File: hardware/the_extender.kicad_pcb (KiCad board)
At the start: 4 copper layers, 51.2 x 50.9 mm, 119 parts, among them J0 U262-241N-4BV60, J1 USB_C_Receptacle_USB2.0, J2 U231-091N-3BLRC11, J3 PJ-3136-B, J4 PJ-3136-B, J5 AF 10.0 HC6.3, Q1 SSM3J332R,LF, Q2 SSM3J332R,LF, Q3 Q_PNP_CBE, Q4 SSM3J332R,LF, U0 RT6150BGQW, U1 IP5310, U2 RP2040, U3 W25Q32JVSS, U4 FUSB302BMPX, U5 USB2514B_Bi, U6 HS-100B, Y1 ABLS-12.000MHZ-20-B-3-H-T

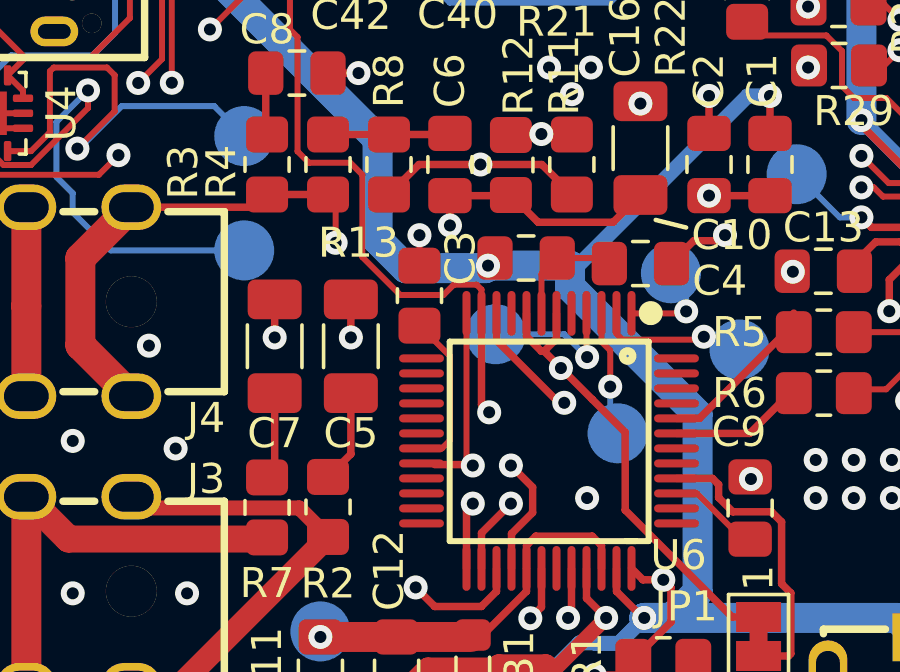
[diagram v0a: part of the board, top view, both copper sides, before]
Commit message: stuff
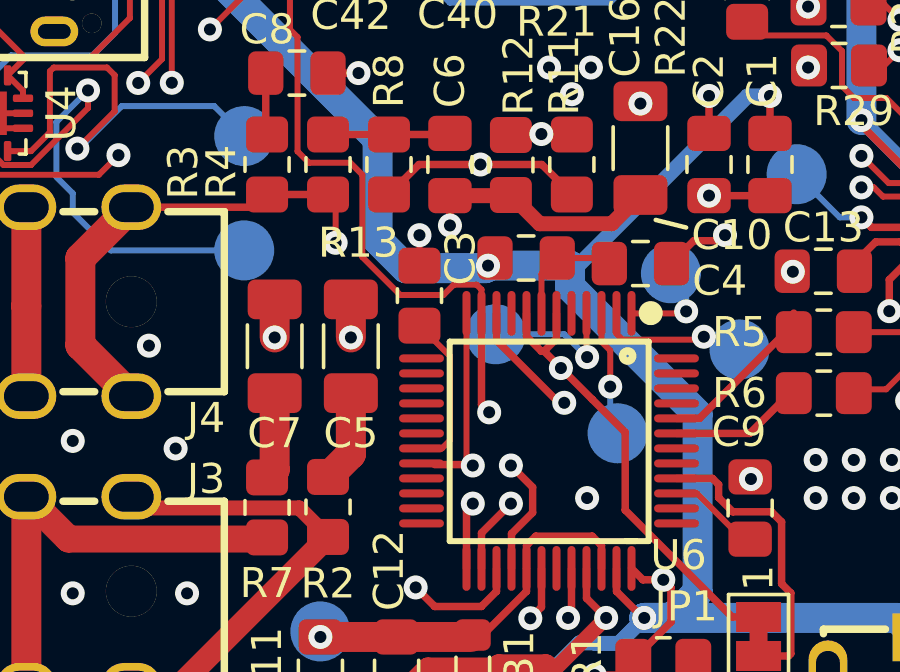
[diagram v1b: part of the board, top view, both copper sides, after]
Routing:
- net Net-(C10-Pad1): track 24.1 -> 26.4 mm
- net SND_L: track 16.0 -> 16.6 mm
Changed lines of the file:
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@@
   (segment (start 69.215 69.4) (end 69.33 69.285) (width 0.25) (layer "F.Cu") (net 5))
   (segment (start 69.33 69.285) (end 69.33 67.75) (width 0.25) (layer "F.Cu") (net 5))
-  (segment (start 61.976 60.052) (end 61.976 58.782) (width 0.25) (layer "F.Cu") (net 5))
+  (segment (start 61.976 60.052) (end 61.976 58.782) (width 1) (layer "F.Cu") (net 5))
   (via (at 61.976 60.052) (size 0.8) (drill 0.4) (layers "F.Cu" "B.Cu") (free) (net 5))
   (via (at 69.215 69.4) (size 0.8) (drill 0.4) (layers "F.Cu" "B.Cu") (free) (net 5))
-  (segment (start 67.116386 67.691) (end 68.58 67.691) (width 0.25) (layer "In1.Cu") (net 5))
-  (segment (start 61.976 60.052) (end 61.976 62.550614) (width 0.25) (layer "In1.Cu") (net 5))
-  (segment (start 68.58 67.691) (end 69.215 68.326) (width 0.25) (layer "In1.Cu") (net 5))
-  (segment (start 69.215 68.326) (end 69.215 69.4) (width 0.25) (layer "In1.Cu") (net 5))
-  (segment (start 61.976 62.550614) (end 67.116386 67.691) (width 0.25) (layer "In1.Cu") (net 5))
-  (segment (start 61.976 61.907) (end 61.976 63.939) (width 0.25) (layer "F.Cu") (net 6))
-  (segment (start 61.976 63.939) (end 61.214 64.701) (width 0.25) (layer "F.Cu") (net 6))
+  (segment (start 68.072 68.199) (end 69.215 69.342) (width 0.5) (layer "In1.Cu") (net 5))
+  (segment (start 66.929 68.199) (end 68.072 68.199) (width 0.5) (layer "In1.Cu") (net 5))
+  (segment (start 61.976 60.052) (end 61.976 63.246) (width 0.5) (layer "In1.Cu") (net 5))
+  (segment (start 61.976 63.246) (end 66.929 68.199) (width 0.5) (layer "In1.Cu") (net 5))
+  (segment (start 69.215 69.342) (end 69.215 69.4) (width 0.5) (layer "In1.Cu") (net 5))
+  (segment (start 61.976 61.907) (end 61.976 63.939) (width 1) (layer "F.Cu") (net 6))
+  (segment (start 61.976 63.939) (end 61.214 64.701) (width 1) (layer "F.Cu") (net 6))
   (segment (start 63.5 72.11) (end 64.5408 71.0692) (width 0.7) (layer "F.Cu") (net 7))
-  (segment (start 65.278 55.3245) (end 67.2885 55.3245) (width 0.25) (layer "F.Cu") (net 7))
+  (segment (start 70.67 56.261) (end 68.268 56.261) (width 0.5) (layer "F.Cu") (net 7))
+  (segment (start 65.278 55.3245) (end 67.2885 55.3245) (width 0.5) (layer "F.Cu") (net 7))
   (segment (start 66.905512 70.96348) (end 68.47848 70.96348) (width 0.7) (layer "F.Cu") (net 7))
   (segment (start 65.83 65.8) (end 65.83 67.75) (width 0.25) (layer "F.Cu") (net 7))
-  (segment (start 67.2885 55.3245) (end 67.31 55.303) (width 0.25) (layer "F.Cu") (net 7))
+  (segment (start 67.2885 55.3245) (end 67.31 55.303) (width 1) (layer "F.Cu") (net 7))
   (segment (start 47.958 62.009) (end 47.912 62.009) (width 1) (layer "F.Cu") (net 7))
   (segment (start 47.912 62.009) (end 46.958479 61.055479) (width 1) (layer "F.Cu") (net 7))
   (segment (start 68.7 71.185) (end 68.7 72.575) (width 0.5) (layer "F.Cu") (net 7))
   (segment (start 60.96 72.11) (end 63.5 72.11) (width 1) (layer "F.Cu") (net 7))
-  (segment (start 68.21852 56.21152) (end 67.31 55.303) (width 0.25) (layer "F.Cu") (net 7))
   (segment (start 49.322 73.025) (end 60.045 73.025) (width 0.75) (layer "F.Cu") (net 7))
   (segment (start 69.83 67.75) (end 69.83 68.745) (width 0.25) (layer "F.Cu") (net 7))
@@
   (segment (start 46.958479 66.360521) (end 46.958479 70.661479) (width 1) (layer "F.Cu") (net 7))
   (segment (start 47.958 71.661) (end 49.322 73.025) (width 0.75) (layer "F.Cu") (net 7))
-  (segment (start 71.628 55.303) (end 70.71948 56.21152) (width 0.25) (layer "F.Cu") (net 7))
   (segment (start 47.958 65.361) (end 47.958 62.009) (width 1) (layer "F.Cu") (net 7))
   (segment (start 66.04 65.59) (end 65.83 65.8) (width 0.25) (layer "F.Cu") (net 7))
@@
   (segment (start 64.5408 71.0692) (end 66.799792 71.0692) (width 0.7) (layer "F.Cu") (net 7))
   (segment (start 47.958 65.361) (end 46.958479 66.360521) (width 1) (layer "F.Cu") (net 7))
+  (segment (start 71.628 55.303) (end 70.67 56.261) (width 0.5) (layer "F.Cu") (net 7))
   (segment (start 46.958479 70.661479) (end 47.958 71.661) (width 1) (layer "F.Cu") (net 7))
+  (segment (start 68.268 56.261) (end 67.31 55.303) (width 0.5) (layer "F.Cu") (net 7))
   (segment (start 46.958479 61.055479) (end 46.958479 56.708521) (width 1) (layer "F.Cu") (net 7))
   (segment (start 60.045 73.025) (end 60.96 72.11) (width 0.75) (layer "F.Cu") (net 7))
   (segment (start 66.799792 71.0692) (end 66.905512 70.96348) (width 0.7) (layer "F.Cu") (net 7))
   (segment (start 65.278 56.319) (end 65.278 55.3245) (width 0.25) (layer "F.Cu") (net 7))
-  (segment (start 70.71948 56.21152) (end 68.21852 56.21152) (width 0.25) (layer "F.Cu") (net 7))
   (via (at 65.278 56.319) (size 0.8) (drill 0.4) (layers "F.Cu" "B.Cu") (free) (net 7))
   (via (at 66.04 65.59) (size 0.8) (drill 0.4) (layers "F.Cu" "B.Cu") (free) (net 7))
@@
   (segment (start 61.214 53.287) (end 63.246 53.287) (width 0.25) (layer "F.Cu") (net 8))
   (segment (start 63.246 53.287) (end 65.2405 53.287) (width 0.25) (layer "F.Cu") (net 8))
-  (segment (start 59.436 60.052) (end 59.436 58.782) (width 0.25) (layer "F.Cu") (net 9))
+  (segment (start 59.436 60.052) (end 59.436 58.782) (width 1) (layer "F.Cu") (net 9))
   (segment (start 68.33 69.039458) (end 68.33 67.75) (width 0.25) (layer "F.Cu") (net 9))
   (segment (start 67.957229 69.412229) (end 68.33 69.039458) (width 0.25) (layer "F.Cu") (net 9))
   (via (at 67.957229 69.412229) (size 0.8) (drill 0.4) (layers "F.Cu" "B.Cu") (free) (net 9))
   (via (at 59.436 60.052) (size 0.8) (drill 0.4) (layers "F.Cu" "B.Cu") (free) (net 9))
-  (segment (start 67.957229 69.354229) (end 67.957229 69.412229) (width 0.25) (layer "In1.Cu") (net 9))
-  (segment (start 59.436 60.833) (end 67.957229 69.354229) (width 0.25) (layer "In1.Cu") (net 9))
-  (segment (start 59.436 60.052) (end 59.436 60.833) (width 0.25) (layer "In1.Cu") (net 9))
-  (segment (start 59.436 64.463) (end 59.182 64.717) (width 0.25) (layer "F.Cu") (net 10))
-  (segment (start 59.436 61.907) (end 59.436 64.463) (width 0.25) (layer "F.Cu") (net 10))
+  (segment (start 59.436 60.052) (end 59.436 61.976) (width 0.5) (layer "In1.Cu") (net 9))
+  (segment (start 59.436 61.976) (end 66.872229 69.412229) (width 0.5) (layer "In1.Cu") (net 9))
+  (segment (start 66.872229 69.412229) (end 67.957229 69.412229) (width 0.5) (layer "In1.Cu") (net 9))
+  (segment (start 59.436 64.463) (end 59.182 64.717) (width 1) (layer "F.Cu") (net 10))
+  (segment (start 59.436 61.907) (end 59.436 64.463) (width 1) (layer "F.Cu") (net 10))
   (segment (start 59.139 51.239) (end 59.139 53.244) (width 0.25) (layer "F.Cu") (net 11))
   (segment (start 59.139 53.244) (end 59.182 53.287) (width 0.25) (layer "F.Cu") (net 11))
@@
   (via (at 71.628 52.255) (size 0.8) (drill 0.4) (layers "F.Cu" "B.Cu") (net 13))
   (via (at 64.135 68.384) (size 0.8) (drill 0.4) (layers "F.Cu" "B.Cu") (net 13))
-  (segment (start 64.135 68.384) (end 65.540614 68.384) (width 0.25) (layer "In2.Cu") (net 13))
-  (segment (start 71.628 62.296614) (end 71.628 52.255) (width 0.25) (layer "In2.Cu") (net 13))
-  (segment (start 65.540614 68.384) (end 71.628 62.296614) (width 0.25) (layer "In2.Cu") (net 13))
+  (segment (start 70.231 67.31) (end 67.564 67.31) (width 1) (layer "In2.Cu") (net 13))
+  (segment (start 71.628 52.255) (end 71.882 52.509) (width 1) (layer "In2.Cu") (net 13))
+  (segment (start 71.882 52.509) (end 71.882 65.659) (width 1) (layer "In2.Cu") (net 13))
+  (segment (start 66.49 68.384) (end 64.135 68.384) (width 1) (layer "In2.Cu") (net 13))
+  (segment (start 67.564 67.31) (end 66.49 68.384) (width 1) (layer "In2.Cu") (net 13))
+  (segment (start 71.882 65.659) (end 70.231 67.31) (width 1) (layer "In2.Cu") (net 13))
   (segment (start 79.473125 56.864489) (end 78.7615 57.576114) (width 0.25) (layer "F.Cu") (net 14))
   (segment (start 78.7615 57.576114) (end 78.7615 57.843) (width 0.25) (layer "F.Cu") (net 14))

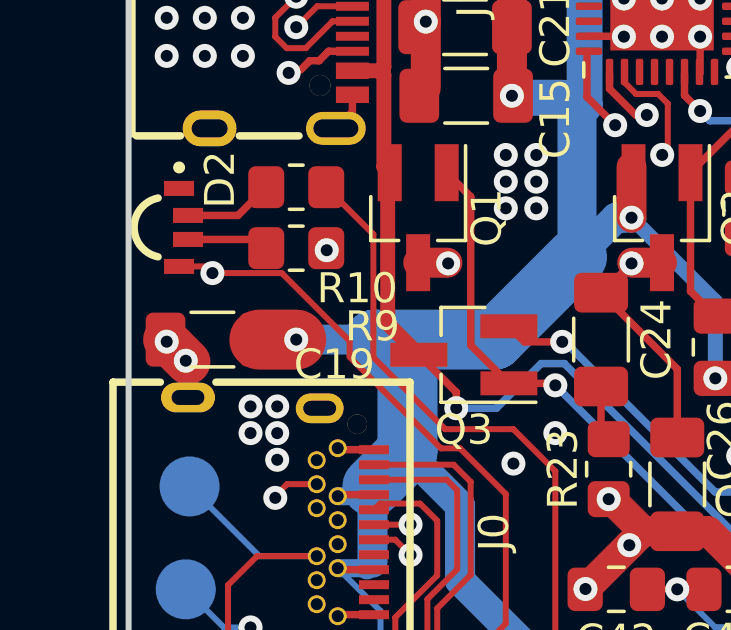
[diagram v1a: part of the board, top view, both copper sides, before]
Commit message: fix
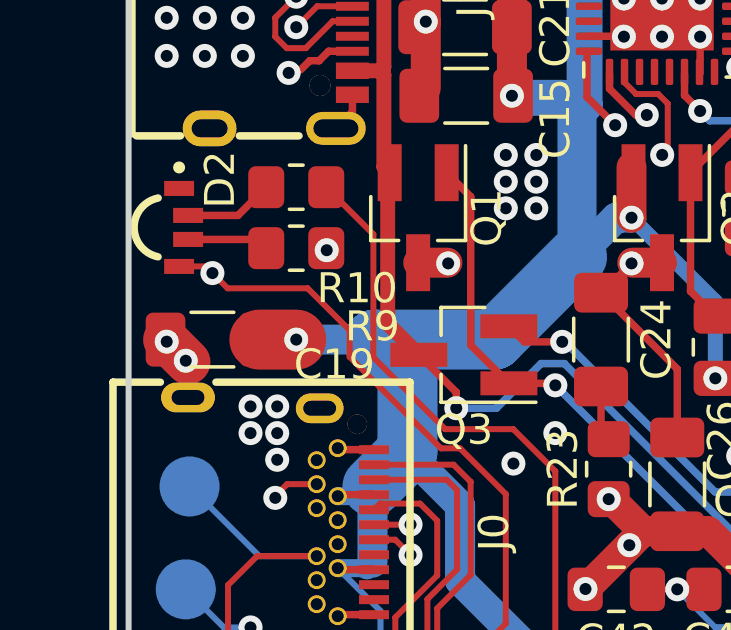
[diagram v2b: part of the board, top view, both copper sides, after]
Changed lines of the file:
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@@
   (segment (start 69.63042 62.77242) (end 69.088 62.23) (width 0.2) (layer "In1.Cu") (net 125))
   (segment (start 82.13458 53.88242) (end 81.82242 54.19458) (width 0.2) (layer "In1.Cu") (net 125))
+  (segment (start 48.514 37.084) (end 49.022 37.592) (width 0.2) (layer "F.Cu") (net 145))
   (segment (start 48.292 36.862) (end 48.514 37.084) (width 0.2) (layer "F.Cu") (net 145))
+  (segment (start 53.086 39.878) (end 56.134 42.926) (width 0.2) (layer "F.Cu") (net 145))
   (segment (start 47.4026 36.862) (end 48.292 36.862) (width 0.2) (layer "F.Cu") (net 145))
+  (segment (start 56.134 42.926) (end 56.769 42.926) (width 0.2) (layer "F.Cu") (net 145))
+  (segment (start 49.022 37.592) (end 51.689 37.592) (width 0.2) (layer "F.Cu") (net 145))
+  (segment (start 51.689 37.592) (end 53.086 38.989) (width 0.2) (layer "F.Cu") (net 145))
+  (segment (start 64.262 56.642) (end 64.262 57.658) (width 0.2) (layer "F.Cu") (net 145))
   (segment (start 58.293 44.45) (end 58.293 48.768) (width 0.2) (layer "F.Cu") (net 145))
-  (segment (start 53.086 39.344439) (end 53.086 39.878) (width 0.2) (layer "F.Cu") (net 145))
-  (segment (start 56.134 42.926) (end 56.769 42.926) (width 0.2) (layer "F.Cu") (net 145))
-  (segment (start 64.262 56.642) (end 64.262 57.658) (width 0.2) (layer "F.Cu") (net 145))
-  (segment (start 50.825561 37.084) (end 53.086 39.344439) (width 0.2) (layer "F.Cu") (net 145))
-  (segment (start 48.514 37.084) (end 50.825561 37.084) (width 0.2) (layer "F.Cu") (net 145))
+  (segment (start 53.086 38.989) (end 53.086 39.878) (width 0.2) (layer "F.Cu") (net 145))
   (segment (start 58.293 48.768) (end 57.277 49.784) (width 0.2) (layer "F.Cu") (net 145))
-  (segment (start 53.086 39.878) (end 56.134 42.926) (width 0.2) (layer "F.Cu") (net 145))
   (segment (start 56.769 42.926) (end 58.293 44.45) (width 0.2) (layer "F.Cu") (net 145))
   (via (at 48.514 37.084) (size 0.8) (drill 0.4) (layers "F.Cu" "B.Cu") (free) (net 145))
